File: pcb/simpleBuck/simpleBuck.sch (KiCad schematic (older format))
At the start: 24 parts, among them J1 Conn_01x08, J3 Conn_01x04, J4 Conn_01x02, J5 Conn_01x04, J6 Conn_01x02, U1 ANALOG_LTC1288CS8#PBF, U5 TI_LM4040C41IDBZT, U6 TI_DAC122S085CIMM_NOPB

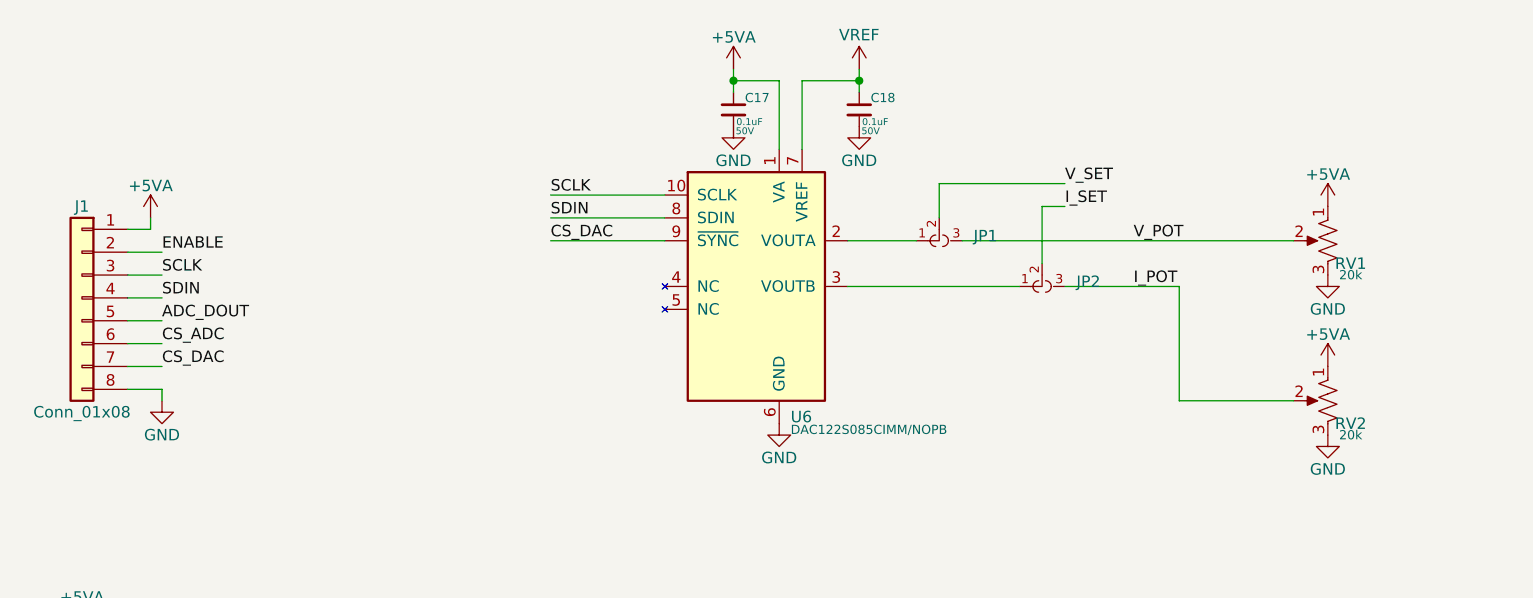
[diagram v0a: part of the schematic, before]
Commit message: Prelim Layout before silkscreen tuning.
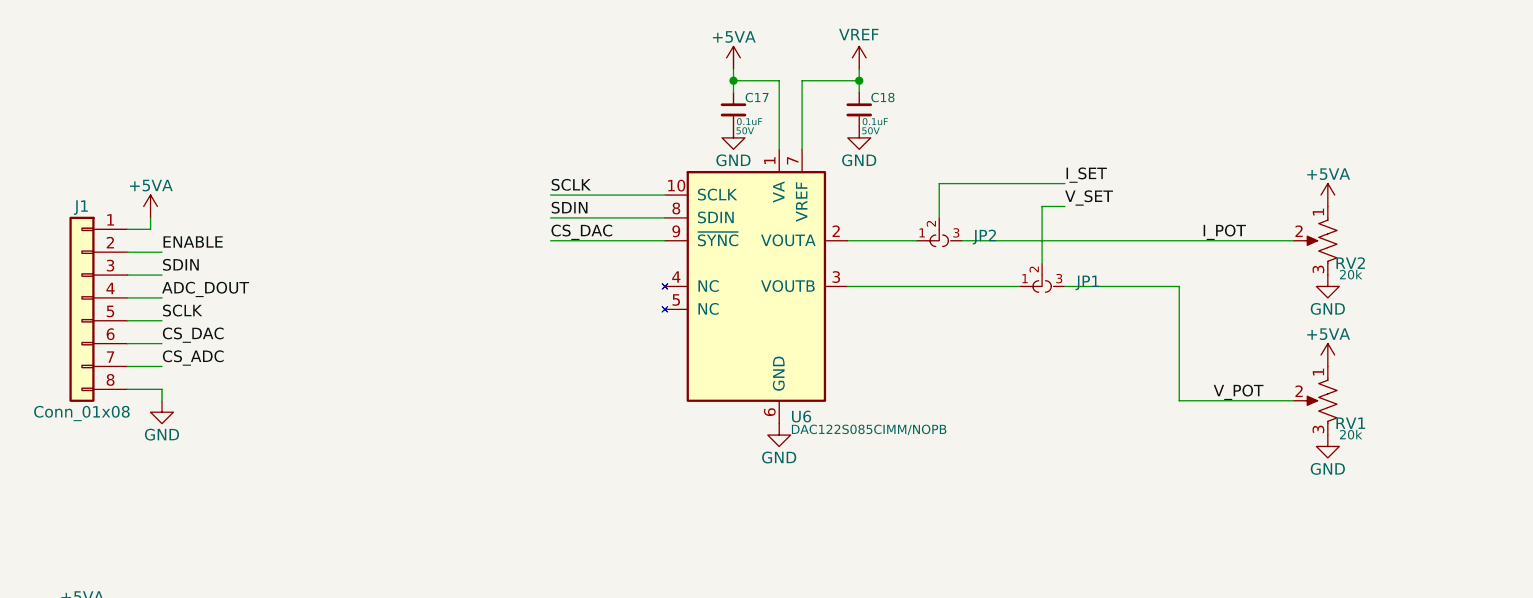
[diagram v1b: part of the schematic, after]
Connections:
- net ADC_DOUT: now also J1.4 (Pin_4); no longer J1.5 (Pin_5)
- net CS_ADC: now also J1.7 (Pin_7); no longer J1.6 (Pin_6)
- net CS_DAC: now also J1.6 (Pin_6); no longer J1.7 (Pin_7)
- net SCLK: now also J1.5 (Pin_5); no longer J1.3 (Pin_3)
- net SDIN: now also J1.3 (Pin_3); no longer J1.4 (Pin_4)
- net at U6.2 (VOUTA): now also JP2.1; no longer JP1.1
- net at U6.3 (VOUTB): now also JP1.1; no longer JP2.1
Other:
- moved on the sheet: JP1, JP2, RV1, RV2
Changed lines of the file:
@@
 Connection ~ 3900 4100
 Connection ~ 4450 4100
-Text Label 1400 5050 0    50   ~ 0
+Text Label 1400 4950 0    50   ~ 0
 SDIN
-Text Label 1400 4950 0    50   ~ 0
+Text Label 1400 5150 0    50   ~ 0
 SCLK
 Text Label 1400 4850 0    50   ~ 0
@@
 Wire Wire Line
 	1250 4850 1400 4850
-Text Label 5350 4550 0    50   ~ 0
-V_SET
 Wire Wire Line
 	1250 5050 1400 5050
@@
 $EndComp
 $Comp
-L DBLS_Resistor:BOURNS_PV37W203C01B00 RV1
-U 1 1 6260CC0E
+L power:GND #PWR036
+U 1 1 6260CC1A
+P 6500 5650
+AR Path="/6260CC1A" Ref="#PWR036"  Part="1"
+AR Path="/620BD2D9/6260CC1A" Ref="#PWR?"  Part="1"
+AR Path="/625BEFFF/6260CC1A" Ref="#PWR?"  Part="1"
+F 0 "#PWR036" H 6500 5400 50  0001 C CNN
+F 1 "GND" H 6500 5500 50  0000 C CNN
+F 2 "" H 6500 5650 50  0001 C CNN
+F 3 "" H 6500 5650 50  0001 C CNN
+	1    6500 5650
+	1    0    0    -1
+$EndComp
+$Comp
+L DBLS_Resistor:BOURNS_PV37W203C01B00 RV2
+U 1 1 62616BEB
 P 6500 4800
-AR Path="/6260CC0E" Ref="RV1"  Part="1"
-AR Path="/625BEFFF/6260CC0E" Ref="RV?"  Part="1"
-F 0 "RV1" H 6400 4700 50  0000 C CNN
+AR Path="/62616BEB" Ref="RV2"  Part="1"
+AR Path="/625BEFFF/62616BEB" Ref="RV?"  Part="1"
+F 0 "RV2" H 6400 4700 50  0000 C CNN
 F 1 "BOURNS_PV37W203C01B00" V 6400 4800 50  0001 C CNN
 F 2 "Potentiometers:Potentiometer_Trimmer_Bourns_3299Y" H 6500 4800 50  0001 C CNN
@@
 $Comp
 L power:+5VA #PWR?
-U 1 1 6260CC14
+U 1 1 62616BF1
 P 6500 4650
-AR Path="/620BD2D9/6260CC14" Ref="#PWR?"  Part="1"
-AR Path="/6260CC14" Ref="#PWR031"  Part="1"
-AR Path="/625BEFFF/6260CC14" Ref="#PWR?"  Part="1"
-F 0 "#PWR031" H 6500 4500 50  0001 C CNN
+AR Path="/620BD2D9/62616BF1" Ref="#PWR?"  Part="1"
+AR Path="/62616BF1" Ref="#PWR037"  Part="1"
+AR Path="/625BEFFF/62616BF1" Ref="#PWR?"  Part="1"
+F 0 "#PWR037" H 6500 4500 50  0001 C CNN
 F 1 "+5VA" H 6500 4790 50  0000 C CNN
 F 2 "" H 6500 4650 50  0001 C CNN
@@
 $EndComp
 $Comp
-L power:GND #PWR036
-U 1 1 6260CC1A
+L power:GND #PWR048
+U 1 1 62616BF7
 P 6500 4950
-AR Path="/6260CC1A" Ref="#PWR036"  Part="1"
-AR Path="/620BD2D9/6260CC1A" Ref="#PWR?"  Part="1"
-AR Path="/625BEFFF/6260CC1A" Ref="#PWR?"  Part="1"
-F 0 "#PWR036" H 6500 4700 50  0001 C CNN
+AR Path="/62616BF7" Ref="#PWR048"  Part="1"
+AR Path="/620BD2D9/62616BF7" Ref="#PWR?"  Part="1"
+AR Path="/625BEFFF/62616BF7" Ref="#PWR?"  Part="1"
+F 0 "#PWR048" H 6500 4700 50  0001 C CNN
 F 1 "GND" H 6500 4800 50  0000 C CNN
 F 2 "" H 6500 4950 50  0001 C CNN
@@
 	1    0    0    -1
 $EndComp
-$Comp
-L DBLS_Misc:PAD_JUMPER_3PIN_12_NC_BY_TRACE JP1
-U 1 1 6260EEAC
-P 4800 4800
-F 0 "JP1" H 4950 4750 50  0000 L BNN
-F 1 "PAD_JUMPER_3PIN_12_NC_BY_TRACE" H 4850 4500 50  0001 C CNN
-F 2 "DBLS_Jumpers:PAD_JUMPER_3PIN_12_NC_BY_TRACE" H 4800 5000 50  0001 C CNN
-F 3 "" H 4800 5000 50  0001 C CNN
-F 4 "DNI" H 5000 4550 25  0001 C CNN "place"
-	1    4800 4800
-	1    0    0    1
-$EndComp
-$Comp
-L DBLS_Resistor:BOURNS_PV37W203C01B00 RV2
-U 1 1 62616BEB
-P 6500 5500
-AR Path="/62616BEB" Ref="RV2"  Part="1"
-AR Path="/625BEFFF/62616BEB" Ref="RV?"  Part="1"
-F 0 "RV2" H 6400 5400 50  0000 C CNN
-F 1 "BOURNS_PV37W203C01B00" V 6400 5500 50  0001 C CNN
-F 2 "Potentiometers:Potentiometer_Trimmer_Bourns_3299Y" H 6500 5500 50  0001 C CNN
-F 3 "https://www.bourns.com/docs/Product-Datasheets/pv37.pdf" H 6500 5500 50  0001 C CNN
-F 4 "Bourns Inc" H 6500 5500 50  0001 C CNN "mfg"
-F 5 "PV37W203C01B00" H 6500 5500 50  0001 C CNN "mfg_pn"
-F 6 "digikey" H 6500 5500 50  0001 C CNN "vendor"
-F 7 "490-2976-ND" H 6500 5500 50  0001 C CNN "vendor_pn"
-F 8 "yes" H 6500 5500 50  0001 C CNN "place"
-F 9 "20k" H 6400 5350 40  0000 C CNN "resistance"
-F 10 "TRIMMER 20K OHM 0.25W PC PIN TOP" H 6500 5500 50  0001 C CNN "description"
-	1    6500 5500
-	-1   0    0    -1
-$EndComp
-$Comp
-L power:+5VA #PWR?
-U 1 1 62616BF1
-P 6500 5350
-AR Path="/620BD2D9/62616BF1" Ref="#PWR?"  Part="1"
-AR Path="/62616BF1" Ref="#PWR037"  Part="1"
-AR Path="/625BEFFF/62616BF1" Ref="#PWR?"  Part="1"
-F 0 "#PWR037" H 6500 5200 50  0001 C CNN
-F 1 "+5VA" H 6500 5490 50  0000 C CNN
-F 2 "" H 6500 5350 50  0001 C CNN
-F 3 "" H 6500 5350 50  0001 C CNN
-	1    6500 5350
-	1    0    0    -1
-$EndComp
-$Comp
-L power:GND #PWR048
-U 1 1 62616BF7
-P 6500 5650
-AR Path="/62616BF7" Ref="#PWR048"  Part="1"
-AR Path="/620BD2D9/62616BF7" Ref="#PWR?"  Part="1"
-AR Path="/625BEFFF/62616BF7" Ref="#PWR?"  Part="1"
-F 0 "#PWR048" H 6500 5400 50  0001 C CNN
-F 1 "GND" H 6500 5500 50  0000 C CNN
-F 2 "" H 6500 5650 50  0001 C CNN
-F 3 "" H 6500 5650 50  0001 C CNN
-	1    6500 5650
-	1    0    0    -1
-$EndComp
-$Comp
-L DBLS_Misc:PAD_JUMPER_3PIN_12_NC_BY_TRACE JP2
-U 1 1 62617E21
-P 5250 5000
-F 0 "JP2" H 5400 4950 50  0000 L BNN
-F 1 "PAD_JUMPER_3PIN_12_NC_BY_TRACE" H 5300 4700 50  0001 C CNN
-F 2 "DBLS_Jumpers:PAD_JUMPER_3PIN_12_NC_BY_TRACE" H 5250 5200 50  0001 C CNN
-F 3 "" H 5250 5200 50  0001 C CNN
-F 4 "DNI" H 5450 4750 25  0001 C CNN "place"
-	1    5250 5000
-	1    0    0    1
-$EndComp
-Wire Wire Line
-	4700 4800 4400 4800
 Wire Wire Line
 	4400 5000 5150 5000
@@
 Wire Wire Line
 	5850 5500 6350 5500
-Wire Wire Line
-	6350 4800 4900 4800
-Wire Wire Line
-	5250 4900 5250 4650
-Wire Wire Line
-	5250 4650 5350 4650
-Wire Wire Line
-	4800 4700 4800 4550
-Wire Wire Line
-	4800 4550 5350 4550
-Text Label 5350 4650 0    50   ~ 0
-I_SET
-Text Label 5650 4800 0    50   ~ 0
-V_POT
-Text Label 5650 5000 0    50   ~ 0
+Text Label 5950 4800 0    50   ~ 0
 I_POT
 $Comp
@@
 	-1   0    0    -1
 $EndComp
+Text Label 1400 5250 0    50   ~ 0
+CS_DAC
 Text Label 1400 5350 0    50   ~ 0
-CS_DAC
-Text Label 1400 5250 0    50   ~ 0
 CS_ADC
 Wire Wire Line
@@
 Text Label 8100 4900 0    50   ~ 0
 ADC_DOUT
-Text Label 1400 5150 0    50   ~ 0
+Text Label 1400 5050 0    50   ~ 0
 ADC_DOUT
 $Comp
@@
 Wire Wire Line
 	10400 1300 10550 1300
+$Comp
+L DBLS_Misc:PAD_JUMPER_3PIN_12_NC_BY_TRACE JP2
+U 1 1 62617E21
+P 4800 4800
+F 0 "JP2" H 4950 4750 50  0000 L BNN
+F 1 "PAD_JUMPER_3PIN_12_NC_BY_TRACE" H 4850 4500 50  0001 C CNN
+F 2 "DBLS_Jumpers:PAD_JUMPER_3PIN_12_NC_BY_TRACE" H 4800 5000 50  0001 C CNN
+F 3 "" H 4800 5000 50  0001 C CNN
+F 4 "DNI" H 5000 4550 25  0001 C CNN "place"
+	1    4800 4800
+	1    0    0    1
+$EndComp
+$Comp
+L DBLS_Misc:PAD_JUMPER_3PIN_12_NC_BY_TRACE JP1
+U 1 1 6260EEAC
+P 5250 5000
+F 0 "JP1" H 5400 4950 50  0000 L BNN
+F 1 "PAD_JUMPER_3PIN_12_NC_BY_TRACE" H 5300 4700 50  0001 C CNN
+F 2 "DBLS_Jumpers:PAD_JUMPER_3PIN_12_NC_BY_TRACE" H 5250 5200 50  0001 C CNN
+F 3 "" H 5250 5200 50  0001 C CNN
+F 4 "DNI" H 5450 4750 25  0001 C CNN "place"
+	1    5250 5000
+	1    0    0    1
+$EndComp
+Text Label 6000 5500 0    50   ~ 0
+V_POT
+Text Label 5350 4550 0    50   ~ 0
+I_SET
+Wire Wire Line
+	4800 4550 5350 4550
+Wire Wire Line
+	4800 4700 4800 4550
+Wire Wire Line
+	5250 4650 5350 4650
+Wire Wire Line
+	5250 4900 5250 4650
+Wire Wire Line
+	6350 4800 4900 4800
+Wire Wire Line
+	4700 4800 4400 4800
+$Comp
+L power:+5VA #PWR?
+U 1 1 6260CC14
+P 6500 5350
+AR Path="/620BD2D9/6260CC14" Ref="#PWR?"  Part="1"
+AR Path="/6260CC14" Ref="#PWR031"  Part="1"
+AR Path="/625BEFFF/6260CC14" Ref="#PWR?"  Part="1"
+F 0 "#PWR031" H 6500 5200 50  0001 C CNN
+F 1 "+5VA" H 6500 5490 50  0000 C CNN
+F 2 "" H 6500 5350 50  0001 C CNN
+F 3 "" H 6500 5350 50  0001 C CNN
+	1    6500 5350
+	1    0    0    -1
+$EndComp
+$Comp
+L DBLS_Resistor:BOURNS_PV37W203C01B00 RV1
+U 1 1 6260CC0E
+P 6500 5500
+AR Path="/6260CC0E" Ref="RV1"  Part="1"
+AR Path="/625BEFFF/6260CC0E" Ref="RV?"  Part="1"
+F 0 "RV1" H 6400 5400 50  0000 C CNN
+F 1 "BOURNS_PV37W203C01B00" V 6400 5500 50  0001 C CNN
+F 2 "Potentiometers:Potentiometer_Trimmer_Bourns_3299Y" H 6500 5500 50  0001 C CNN
+F 3 "https://www.bourns.com/docs/Product-Datasheets/pv37.pdf" H 6500 5500 50  0001 C CNN
+F 4 "Bourns Inc" H 6500 5500 50  0001 C CNN "mfg"
+F 5 "PV37W203C01B00" H 6500 5500 50  0001 C CNN "mfg_pn"
+F 6 "digikey" H 6500 5500 50  0001 C CNN "vendor"
+F 7 "490-2976-ND" H 6500 5500 50  0001 C CNN "vendor_pn"
+F 8 "yes" H 6500 5500 50  0001 C CNN "place"
+F 9 "20k" H 6400 5350 40  0000 C CNN "resistance"
+F 10 "TRIMMER 20K OHM 0.25W PC PIN TOP" H 6500 5500 50  0001 C CNN "description"
+	1    6500 5500
+	-1   0    0    -1
+$EndComp
+Text Label 5350 4650 0    50   ~ 0
+V_SET
 $EndSCHEMATC

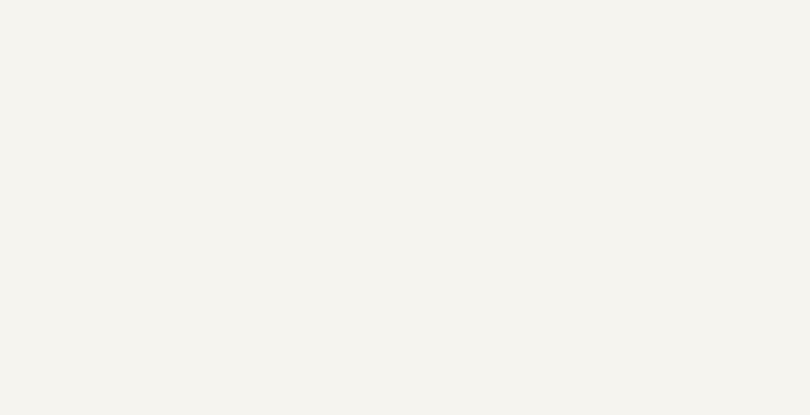
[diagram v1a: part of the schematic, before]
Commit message: Finished layout. Heading to fab
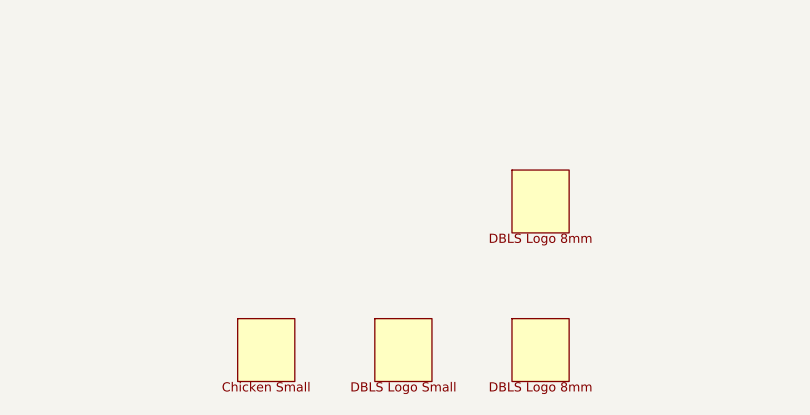
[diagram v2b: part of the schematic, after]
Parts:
- added LOGO1: DBLS_Chicken_Small, DBLS_LOGO:Rooster_4mmx4mm, symbol DBLS_Logo:DBLS_Chicken_Small
- added LOGO2: DBLS_van_logo_small_v1, DBLS_LOGO:van_logo_small, symbol DBLS_Logo:DBLS_van_logo_small_v1
- added LOGO3: DBLS_van_logo_8mmX6mm, DBLS_LOGO:van_logo_8mmX6mm, symbol DBLS_Logo:DBLS_van_logo_8mmX6mm
- added LOGO4: DBLS_van_logo_8mmX6mm_mirror, DBLS_LOGO:van_logo_8mmX6mm_mirror, symbol DBLS_Logo:DBLS_van_logo_8mmX6mm_mirror
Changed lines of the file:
@@
 Text Label 5350 4650 0    50   ~ 0
 V_SET
+$Comp
+L DBLS_Logo:DBLS_van_logo_small_v1 LOGO2
+U 1 1 6287A205
+P 6000 7450
+F 0 "LOGO2" H 6000 7450 50  0001 C CNN
+F 1 "DBLS_van_logo_small_v1" H 6000 7450 50  0001 C CNN
+F 2 "DBLS_LOGO:van_logo_small" H 6030 7600 20  0001 C CNN
+F 3 "" H 6000 7450 50  0001 C CNN
+F 4 "DNI" H 6000 7450 50  0001 C CNN "place"
+	1    6000 7450
+	1    0    0    -1
+$EndComp
+$Comp
+L DBLS_Logo:DBLS_Chicken_Small LOGO1
+U 1 1 6287A7A1
+P 5400 7450
+F 0 "LOGO1" H 5400 7450 50  0001 C CNN
+F 1 "DBLS_Chicken_Small" H 5400 7450 50  0001 C CNN
+F 2 "DBLS_LOGO:Rooster_4mmx4mm" H 5430 7600 20  0001 C CNN
+F 3 "" H 5400 7450 50  0001 C CNN
+F 4 "DNI" H 5400 7450 50  0001 C CNN "place"
+	1    5400 7450
+	1    0    0    -1
+$EndComp
+$Comp
+L DBLS_Logo:DBLS_van_logo_8mmX6mm LOGO3
+U 1 1 62886DDE
+P 6600 7450
+F 0 "LOGO3" H 6600 7450 50  0001 C CNN
+F 1 "DBLS_van_logo_8mmX6mm" H 6600 7450 50  0001 C CNN
+F 2 "DBLS_LOGO:van_logo_8mmX6mm" H 6630 7600 20  0001 C CNN
+F 3 "" H 6600 7450 50  0001 C CNN
+F 4 "DNI" H 6600 7450 50  0001 C CNN "place"
+	1    6600 7450
+	1    0    0    -1
+$EndComp
+$Comp
+L DBLS_Logo:DBLS_van_logo_8mmX6mm_mirror LOGO4
+U 1 1 6289FCE0
+P 6600 6800
+F 0 "LOGO4" H 6600 6800 50  0001 C CNN
+F 1 "DBLS_van_logo_8mmX6mm_mirror" H 6600 6800 50  0001 C CNN
+F 2 "DBLS_LOGO:van_logo_8mmX6mm_mirror" H 6630 6950 20  0001 C CNN
+F 3 "" H 6600 6800 50  0001 C CNN
+F 4 "DNI" H 6600 6800 50  0001 C CNN "place"
+	1    6600 6800
+	1    0    0    -1
+$EndComp
 $EndSCHEMATC
